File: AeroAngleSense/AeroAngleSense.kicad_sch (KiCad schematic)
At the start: 23 parts, among them J1 SM06B-GHS-TBT, J2 SM04B-GHS-TBT, U1 STM32F042F6P6, U2 TPS62842DGRR, U3 TMP127EDBVRQ1

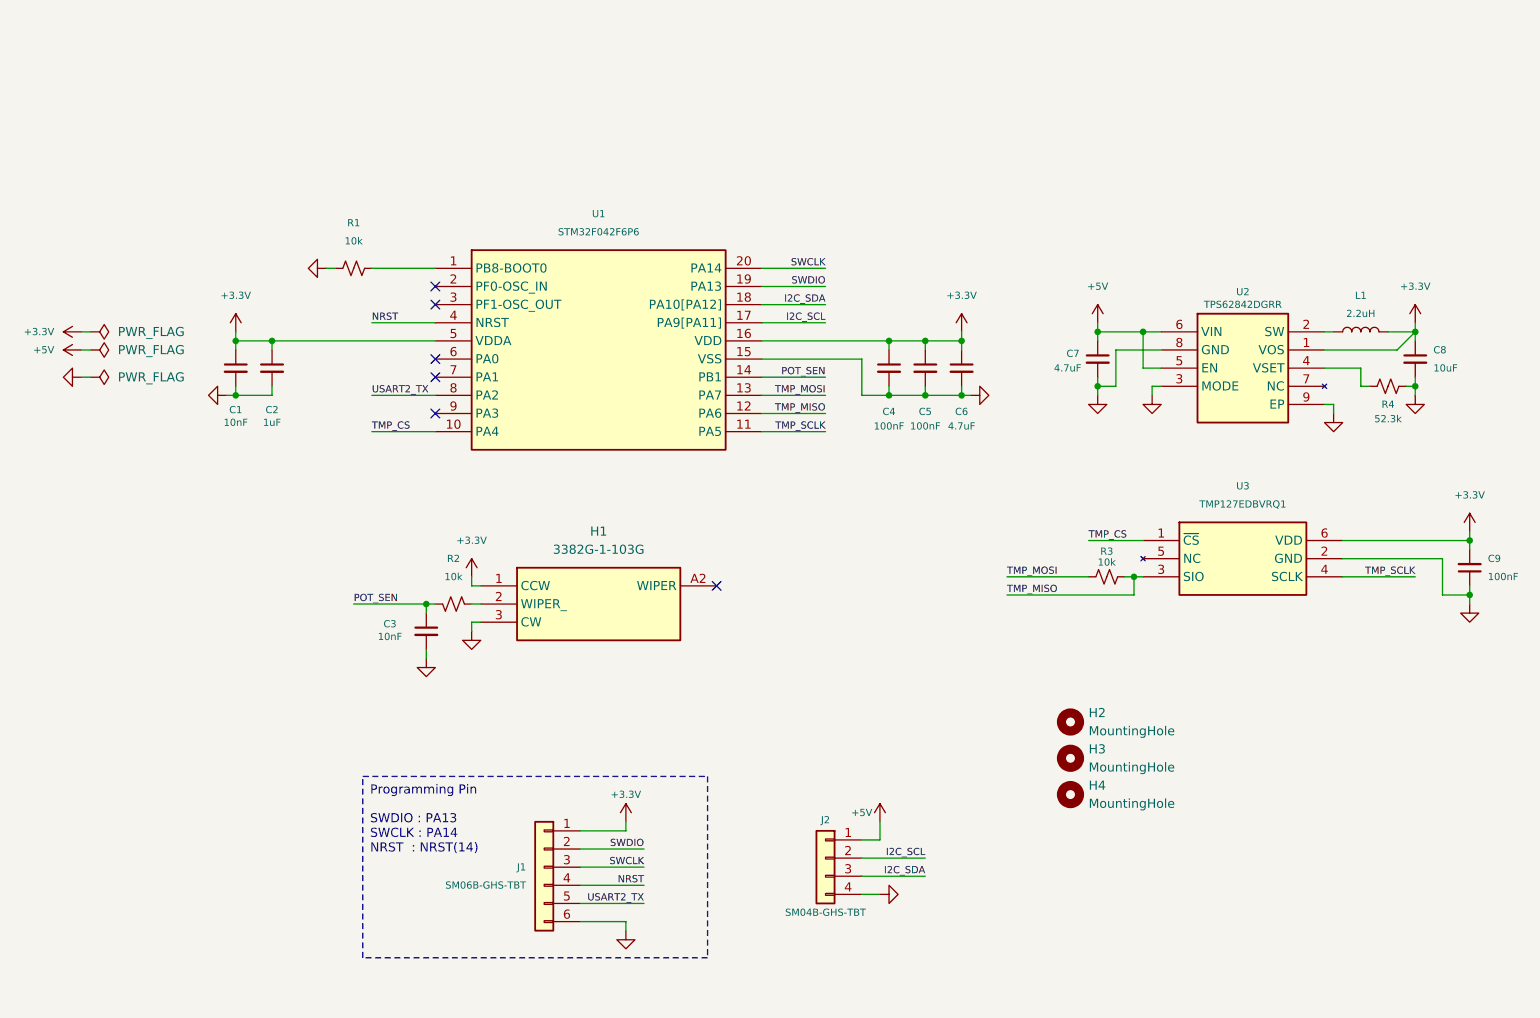
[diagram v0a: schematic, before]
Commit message: fix:readme
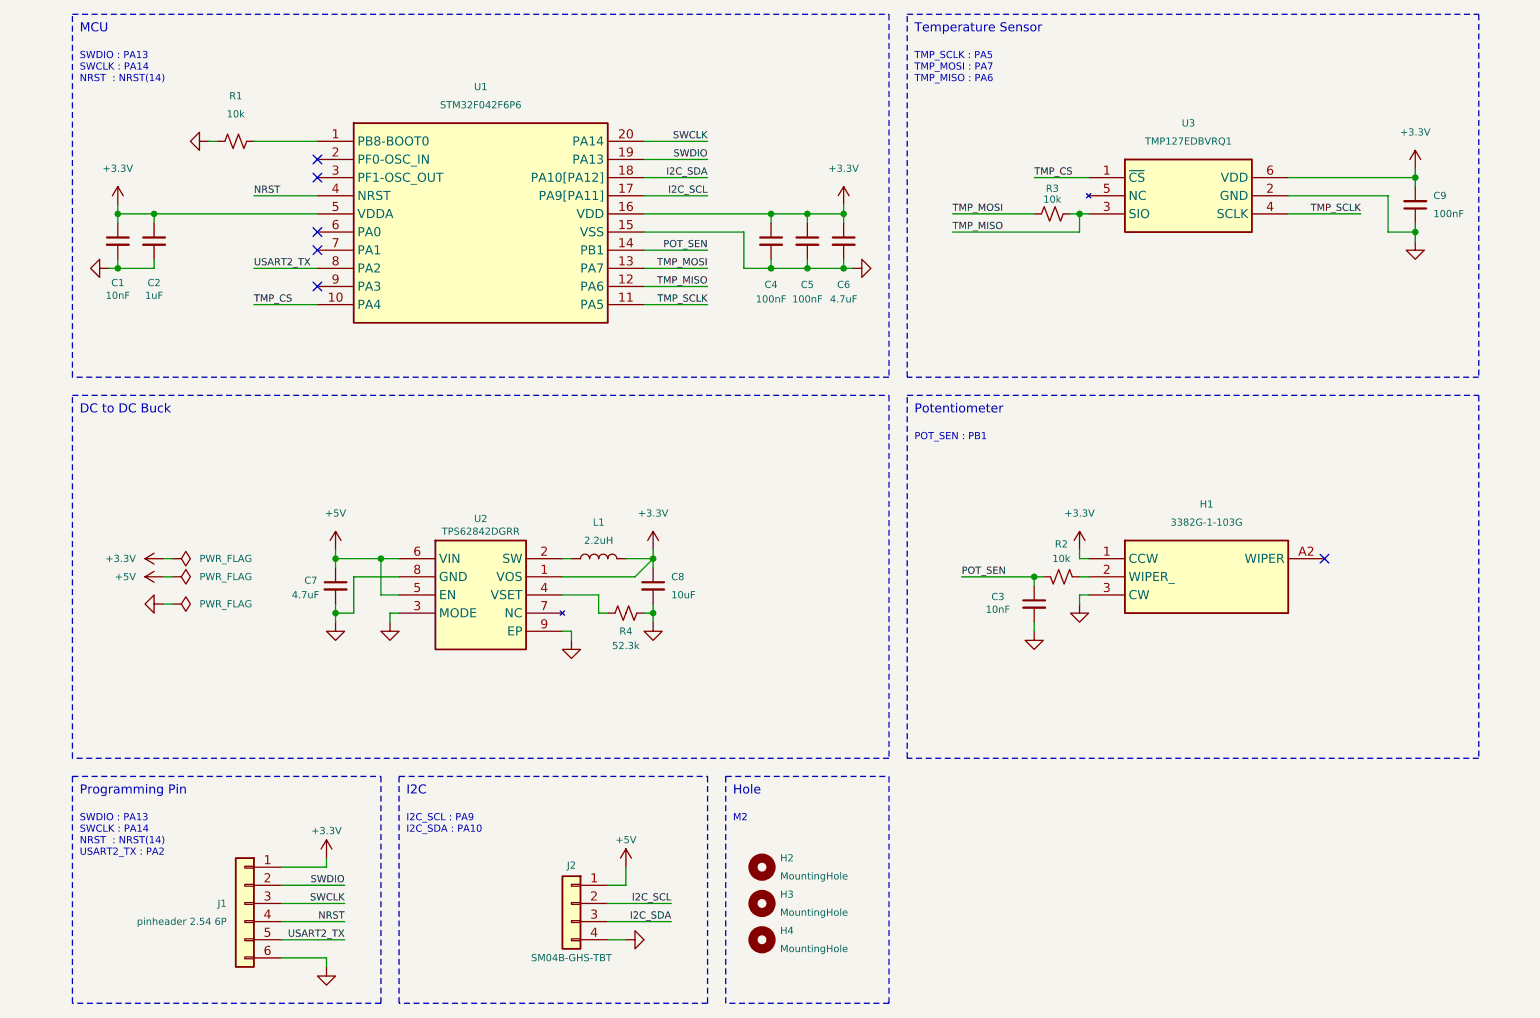
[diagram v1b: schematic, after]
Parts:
- J1: value SM06B-GHS-TBT -> pinheader 2.54 6P; LCSC C133065 -> (none)
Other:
- note added: "DC to DC Buck"
- note added: "Hole"
- note added: "I2C"
- note added: "I2C_SCL : PA9 I2C_SDA : PA10"
- note added: "M2"
- note added: "MCU"
- note added: "POT_SEN : PB1"
- note added: "Potentiometer"
- note added: "SWDIO : PA13 SWCLK : PA14 NRST : NRST(14) USART2_TX : PA2"
- note added: "TMP_SCLK : PA5 TMP_MOSI : PA7 TMP_MISO : PA6"
- note added: "Temperature Sensor"
- company: (none) -> NARAE
- title: (none) -> AeroAngleSense
- moved on the sheet: C1, C2, C3, C4, C5, C6, C7, C8, C9, H1, H2, H3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
